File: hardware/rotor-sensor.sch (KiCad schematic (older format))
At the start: 47 parts, among them J1 Conn_01x03, J2 Conn_01x03, U1 EE-SX199, U2 MCP2021A-xxxxSN, U3 SM351LT, U4 ATtiny202-SS, U5 AP22804AW5

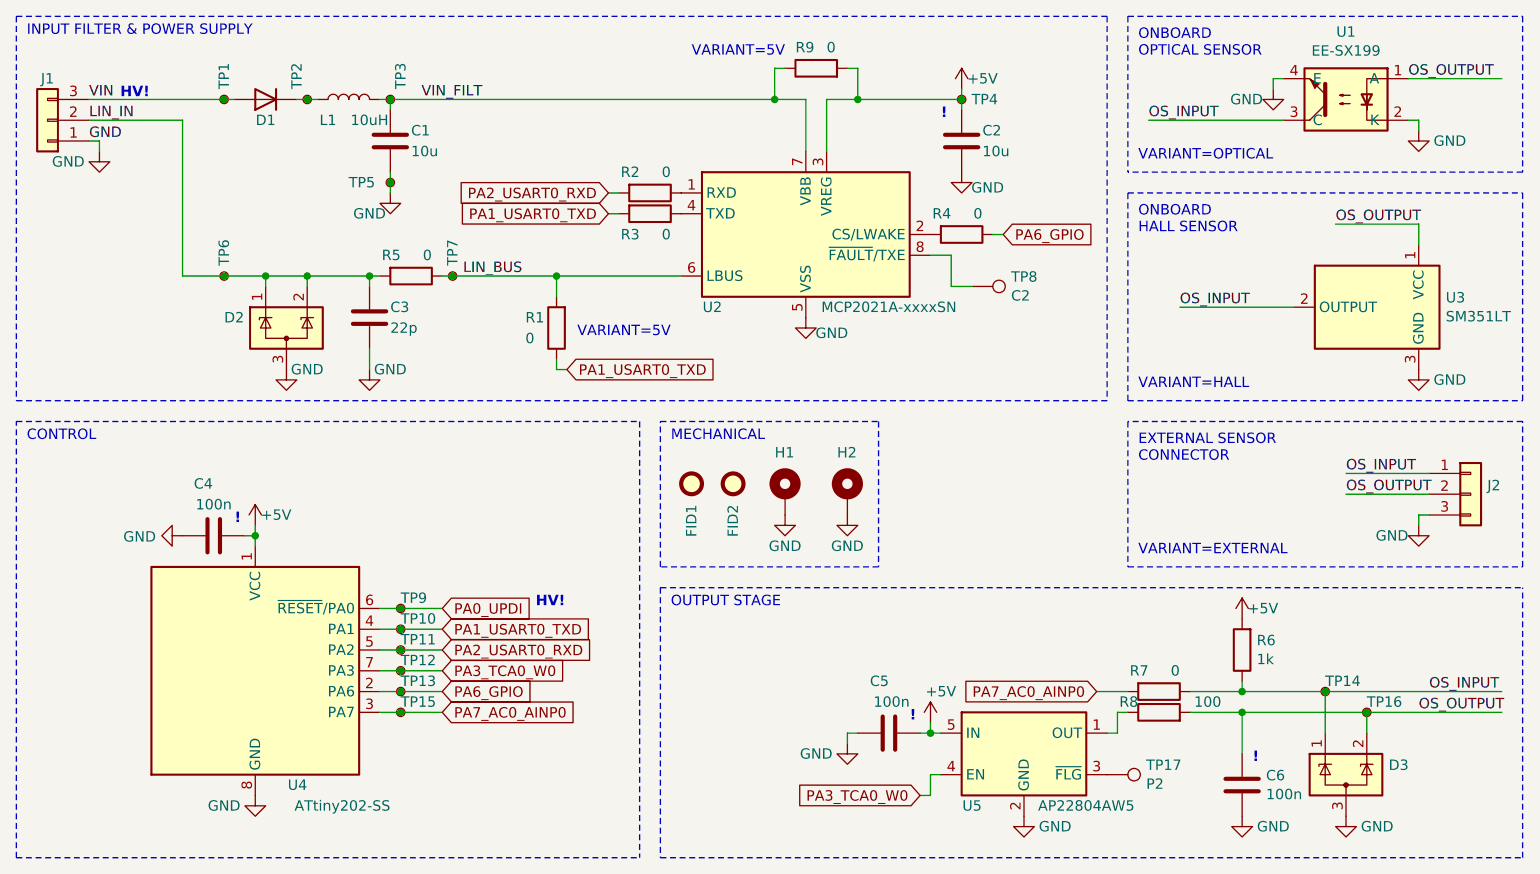
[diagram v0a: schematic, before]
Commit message: Panelize?
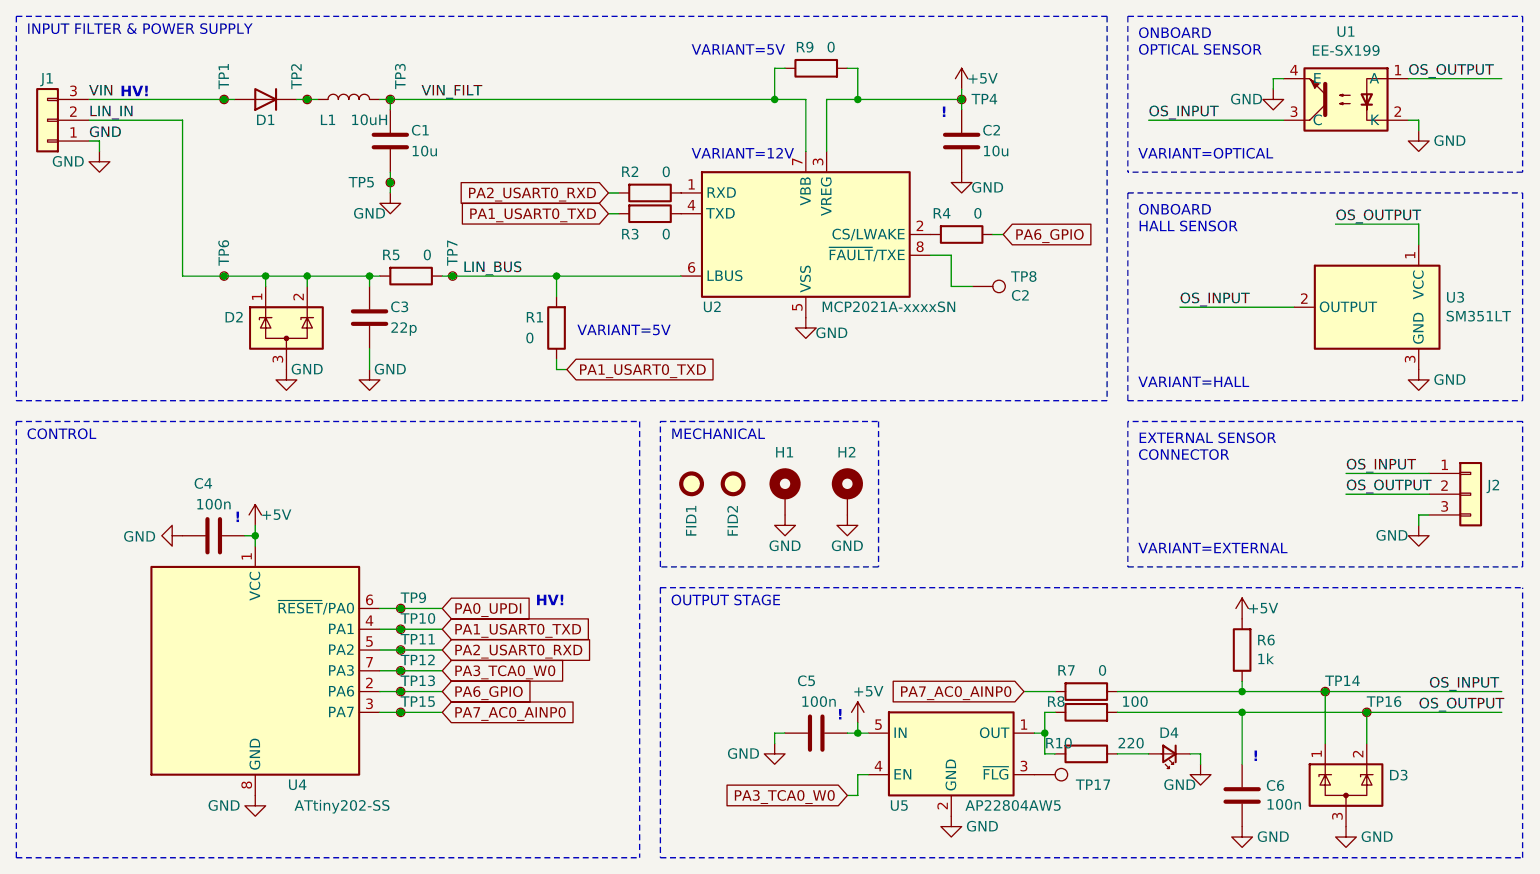
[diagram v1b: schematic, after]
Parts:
- added D4: LED_Small, LED_SMD:LED_0603_1608Metric, symbol Device:LED_Small
- added R10: 220, Resistor_SMD:R_0603_1608Metric, symbol Device:R
- R1, R9: Config (none) -> +5V
- U2: Config (none) -> -5V
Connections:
- wire segments 95 -> 100
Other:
- note added: "VARIANT=12V"
- moved on the sheet: C5, C6, D3, R7, R8, TP17, U5
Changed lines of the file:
@@
 L Device:R R8
 U 1 1 6122E61F
-P 7800 5100
-F 0 "R8" V 7850 5200 50  0000 L CNN
-F 1 "100" V 7850 4800 50  0000 L CNN
-F 2 "Resistor_SMD:R_0603_1608Metric" V 7730 5100 50  0001 C CNN
-F 3 "~" H 7800 5100 50  0001 C CNN
-	1    7800 5100
+P 7450 5100
+F 0 "R8" V 7500 5200 50  0000 L CNN
+F 1 "100" V 7500 4800 50  0000 L CNN
+F 2 "Resistor_SMD:R_0603_1608Metric" V 7380 5100 50  0001 C CNN
+F 3 "~" H 7450 5100 50  0001 C CNN
+	1    7450 5100
 	0    -1   -1   0
 $EndComp
@@
 	-1   0    0    1
 $EndComp
-Text GLabel 7500 5000 0    50   Input ~ 0
+Text GLabel 7150 5000 0    50   Input ~ 0
 PA7_AC0_AINP0
 Wire Wire Line
-	7600 5100 7650 5100
+	7250 5100 7300 5100
 Text GLabel 4350 4700 2    50   Input ~ 0
 PA1_USART0_TXD
@@
 L Power_Protection:SP0502BAHT D3
 U 1 1 613650DD
-P 8700 5400
-F 0 "D3" H 8905 5446 50  0000 L CNN
-F 1 "SP0502BAHT" H 8900 5350 50  0001 L CNN
-F 2 "Package_TO_SOT_SMD:SOT-23" H 8925 5350 50  0001 L CNN
-F 3 "http://www.littelfuse.com/~/media/files/littelfuse/technical%20resources/documents/data%20sheets/sp05xxba.pdf" H 8825 5525 50  0001 C CNN
-	1    8700 5400
+P 8700 5450
+F 0 "D3" H 8905 5496 50  0000 L CNN
+F 1 "SP0502BAHT" H 8900 5400 50  0001 L CNN
+F 2 "Package_TO_SOT_SMD:SOT-23" H 8925 5400 50  0001 L CNN
+F 3 "http://www.littelfuse.com/~/media/files/littelfuse/technical%20resources/documents/data%20sheets/sp05xxba.pdf" H 8825 5575 50  0001 C CNN
+	1    8700 5450
 	1    0    0    -1
 $EndComp
@@
 	8200 4950 8200 5000
 Wire Wire Line
-	8200 5300 8200 5100
+	8200 5350 8200 5100
 $Comp
 L power:GND #PWR024
 U 1 1 613B542D
-P 8700 5600
-F 0 "#PWR024" H 8700 5350 50  0001 C CNN
-F 1 "GND" H 8850 5550 50  0000 C CNN
-F 2 "" H 8700 5600 50  0001 C CNN
-F 3 "" H 8700 5600 50  0001 C CNN
-	1    8700 5600
+P 8700 5650
+F 0 "#PWR024" H 8700 5400 50  0001 C CNN
+F 1 "GND" H 8850 5600 50  0000 C CNN
+F 2 "" H 8700 5650 50  0001 C CNN
+F 3 "" H 8700 5650 50  0001 C CNN
+	1    8700 5650
 	1    0    0    -1
 $EndComp
@@
 L power:GND #PWR023
 U 1 1 6127F551
-P 8200 5600
-F 0 "#PWR023" H 8200 5350 50  0001 C CNN
-F 1 "GND" H 8350 5550 50  0000 C CNN
-F 2 "" H 8200 5600 50  0001 C CNN
-F 3 "" H 8200 5600 50  0001 C CNN
-	1    8200 5600
+P 8200 5650
+F 0 "#PWR023" H 8200 5400 50  0001 C CNN
+F 1 "GND" H 8350 5600 50  0000 C CNN
+F 2 "" H 8200 5650 50  0001 C CNN
+F 3 "" H 8200 5650 50  0001 C CNN
+	1    8200 5650
 	1    0    0    -1
 $EndComp
@@
 L Device:C C6
 U 1 1 61263E24
-P 8200 5450
-F 0 "C6" H 8315 5496 50  0000 L CNN
-F 1 "100n" H 8315 5405 50  0000 L CNN
-F 2 "Capacitor_SMD:C_0603_1608Metric" H 8238 5300 50  0001 C CNN
-F 3 "~" H 8200 5450 50  0001 C CNN
-	1    8200 5450
+P 8200 5500
+F 0 "C6" H 8315 5546 50  0000 L CNN
+F 1 "100n" H 8315 5455 50  0000 L CNN
+F 2 "Capacitor_SMD:C_0603_1608Metric" H 8238 5350 50  0001 C CNN
+F 3 "~" H 8200 5500 50  0001 C CNN
+	1    8200 5500
 	1    0    0    -1
 $EndComp
@@
 OUTPUT STAGE
 Wire Wire Line
-	8200 5000 7950 5000
-Wire Wire Line
-	7650 5000 7500 5000
+	8200 5000 7600 5000
+Wire Wire Line
+	7300 5000 7150 5000
 Text GLabel 4350 4600 2    50   Input ~ 0
 PA0_UPDI
@@
 	8350 2050 8400 2050
 Wire Wire Line
-	8800 5200 8800 5100
+	8800 5250 8800 5100
 Connection ~ 8800 5100
 Wire Wire Line
-	8600 5200 8600 5000
+	8600 5250 8600 5000
 Connection ~ 8600 5000
 Wire Wire Line
@@
 F 2 "Package_SO:SOIC-8_3.9x4.9mm_P1.27mm" H 6125 2875 50  0001 C CNN
 F 3 "http://ww1.microchip.com/downloads/en/DeviceDoc/20002298C.pdf" H 6125 2875 50  0001 C CNN
+F 4 "-5V" H 6100 2800 50  0001 C CNN "Config"
 	1    6100 2800
 	1    0    0    -1
@@
 Text GLabel 4350 4800 2    50   Input ~ 0
 PA2_USART0_RXD
-Wire Wire Line
-	7950 5100 8200 5100
 $Comp
 L Power_Management:AP22804AW5 U5
 U 1 1 623B800F
-P 7150 5300
-F 0 "U5" H 6900 5050 50  0000 C CNN
-F 1 "AP22804AW5" H 7450 5050 50  0000 C CNN
-F 2 "Package_TO_SOT_SMD:SOT-23-5" H 7150 4900 50  0001 C CNN
-F 3 "https://www.diodes.com/assets/Datasheets/AP22804_14.pdf" H 7150 5350 50  0001 C CNN
-	1    7150 5300
+P 6800 5300
+F 0 "U5" H 6550 5050 50  0000 C CNN
+F 1 "AP22804AW5" H 7100 5050 50  0000 C CNN
+F 2 "Package_TO_SOT_SMD:SOT-23-5" H 6800 4900 50  0001 C CNN
+F 3 "https://www.diodes.com/assets/Datasheets/AP22804_14.pdf" H 6800 5350 50  0001 C CNN
+	1    6800 5300
 	1    0    0    -1
 $EndComp
@@
 	5150 2700 5200 2700
 Wire Wire Line
-	7550 5200 7600 5200
-Wire Wire Line
-	7600 5200 7600 5100
+	7200 5200 7250 5200
+Wire Wire Line
+	7250 5200 7250 5100
 Text GLabel 4350 4900 2    50   Input ~ 0
 PA3_TCA0_W0
 Text GLabel 4350 5000 2    50   Input ~ 0
 PA6_GPIO
-Text GLabel 6650 5500 0    50   Input ~ 0
+Text GLabel 6300 5500 0    50   Input ~ 0
 PA3_TCA0_W0
 $Comp
 L power:+5V #PWR019
 U 1 1 623E7E3D
-P 6700 5150
-F 0 "#PWR019" H 6700 5000 50  0001 C CNN
-F 1 "+5V" H 6750 5300 50  0000 C CNN
-F 2 "" H 6700 5150 50  0001 C CNN
-F 3 "" H 6700 5150 50  0001 C CNN
-	1    6700 5150
-	1    0    0    -1
-$EndComp
-Wire Wire Line
-	6700 5400 6750 5400
-Wire Wire Line
-	6700 5150 6700 5200
-Wire Wire Line
-	6700 5200 6750 5200
+P 6350 5150
+F 0 "#PWR019" H 6350 5000 50  0001 C CNN
+F 1 "+5V" H 6400 5300 50  0000 C CNN
+F 2 "" H 6350 5150 50  0001 C CNN
+F 3 "" H 6350 5150 50  0001 C CNN
+	1    6350 5150
+	1    0    0    -1
+$EndComp
+Wire Wire Line
+	6350 5400 6400 5400
+Wire Wire Line
+	6350 5150 6350 5200
+Wire Wire Line
+	6350 5200 6400 5200
 $Comp
 L power:GND #PWR022
 U 1 1 623F4191
-P 7150 5600
-F 0 "#PWR022" H 7150 5350 50  0001 C CNN
-F 1 "GND" H 7300 5550 50  0000 C CNN
-F 2 "" H 7150 5600 50  0001 C CNN
-F 3 "" H 7150 5600 50  0001 C CNN
-	1    7150 5600
+P 6800 5600
+F 0 "#PWR022" H 6800 5350 50  0001 C CNN
+F 1 "GND" H 6950 5550 50  0000 C CNN
+F 2 "" H 6800 5600 50  0001 C CNN
+F 3 "" H 6800 5600 50  0001 C CNN
+	1    6800 5600
 	1    0    0    -1
 $EndComp
@@
 L Device:C C5
 U 1 1 623F6E9E
-P 6500 5200
-F 0 "C5" V 6750 5200 50  0000 L CNN
-F 1 "100n" V 6650 5100 50  0000 L CNN
-F 2 "Capacitor_SMD:C_0603_1608Metric" H 6538 5050 50  0001 C CNN
-F 3 "~" H 6500 5200 50  0001 C CNN
-	1    6500 5200
+P 6150 5200
+F 0 "C5" V 6400 5200 50  0000 L CNN
+F 1 "100n" V 6300 5100 50  0000 L CNN
+F 2 "Capacitor_SMD:C_0603_1608Metric" H 6188 5050 50  0001 C CNN
+F 3 "~" H 6150 5200 50  0001 C CNN
+	1    6150 5200
 	0    -1   -1   0
 $EndComp
@@
 L power:GND #PWR020
 U 1 1 6248AFD5
-P 6300 5250
-F 0 "#PWR020" H 6300 5000 50  0001 C CNN
-F 1 "GND" H 6150 5200 50  0000 C CNN
-F 2 "" H 6300 5250 50  0001 C CNN
-F 3 "" H 6300 5250 50  0001 C CNN
-	1    6300 5250
-	1    0    0    -1
-$EndComp
-Wire Wire Line
-	6650 5500 6700 5500
-Wire Wire Line
-	6700 5500 6700 5400
-Wire Wire Line
-	6300 5250 6300 5200
+P 5950 5250
+F 0 "#PWR020" H 5950 5000 50  0001 C CNN
+F 1 "GND" H 5800 5200 50  0000 C CNN
+F 2 "" H 5950 5250 50  0001 C CNN
+F 3 "" H 5950 5250 50  0001 C CNN
+	1    5950 5250
+	1    0    0    -1
+$EndComp
+Wire Wire Line
+	6300 5500 6350 5500
+Wire Wire Line
+	6350 5500 6350 5400
+Wire Wire Line
+	5950 5250 5950 5200
+Wire Wire Line
+	5950 5200 6000 5200
 Wire Wire Line
 	6300 5200 6350 5200
-Wire Wire Line
-	6650 5200 6700 5200
-Connection ~ 6700 5200
+Connection ~ 6350 5200
 Wire Notes Line
 	5400 4500 9550 4500
@@
 L Device:R R7
 U 1 1 6258FF8B
-P 7800 5000
-F 0 "R7" V 7700 4950 50  0000 R CNN
-F 1 "0" V 7700 5100 50  0000 R CNN
-F 2 "Resistor_SMD:R_0402_1005Metric" V 7730 5000 50  0001 C CNN
-F 3 "~" H 7800 5000 50  0001 C CNN
-	1    7800 5000
+P 7450 5000
+F 0 "R7" V 7350 4950 50  0000 R CNN
+F 1 "0" V 7350 5100 50  0000 R CNN
+F 2 "Resistor_SMD:R_0402_1005Metric" V 7380 5000 50  0001 C CNN
+F 3 "~" H 7450 5000 50  0001 C CNN
+	1    7450 5000
 	0    1    1    0
 $EndComp
@@
 L Connector:TestPoint TP17
 U 1 1 626156D9
-P 7550 5400
-F 0 "TP17" V 7504 5588 50  0000 L CNN
-F 1 "P2" V 7595 5588 50  0000 L CNN
-F 2 "TestPoint:TestPoint_Pad_D1.0mm" H 7750 5400 50  0001 C CNN
-F 3 "~" H 7750 5400 50  0001 C CNN
-	1    7550 5400
+P 7200 5400
+F 0 "TP17" V 7250 5600 50  0000 L CNN
+F 1 "P2" V 7300 5600 50  0001 L CNN
+F 2 "TestPoint:TestPoint_Pad_D1.0mm" H 7400 5400 50  0001 C CNN
+F 3 "~" H 7400 5400 50  0001 C CNN
+	1    7200 5400
 	0    1    1    0
 $EndComp
@@
 Text Label 8650 2750 0    50   ~ 0
 OS_OUTPUT
-Text Notes 6600 5150 0    50   ~ 10
+Text Notes 6250 5150 0    50   ~ 10
 !
 Text Notes 6750 2250 0    50   ~ 10
@@
 F 2 "Resistor_SMD:R_0402_1005Metric" V 4830 3250 50  0001 C CNN
 F 3 "~" H 4900 3250 50  0001 C CNN
+F 4 "+5V" H 4900 3250 50  0001 C CNN "Config"
 	1    4900 3250
 	-1   0    0    1
@@
 F 2 "Resistor_SMD:R_0603_1608Metric" V 6080 2000 50  0001 C CNN
 F 3 "~" H 6150 2000 50  0001 C CNN
+F 4 "+5V" V 6150 2000 50  0001 C CNN "Config"
 	1    6150 2000
 	0    -1   -1   0
@@
 Text Notes 5000 3300 0    50   ~ 0
 VARIANT=5V
+$Comp
+L Device:R R10
+U 1 1 6253E802
+P 7450 5300
+F 0 "R10" V 7400 5100 50  0000 L CNN
+F 1 "220" V 7400 5450 50  0000 L CNN
+F 2 "Resistor_SMD:R_0603_1608Metric" V 7380 5300 50  0001 C CNN
+F 3 "~" H 7450 5300 50  0001 C CNN
+	1    7450 5300
+	0    1    1    0
+$EndComp
+$Comp
+L Device:LED_Small D4
+U 1 1 6253FA73
+P 7850 5300
+F 0 "D4" H 7900 5200 50  0000 R CNN
+F 1 "LED_Small" V 7800 5500 50  0001 R CNN
+F 2 "LED_SMD:LED_0603_1608Metric" V 7850 5300 50  0001 C CNN
+F 3 "~" V 7850 5300 50  0001 C CNN
+	1    7850 5300
+	-1   0    0    1
+$EndComp
+$Comp
+L power:GND #PWR0101
+U 1 1 625403F5
+P 8000 5350
+F 0 "#PWR0101" H 8000 5100 50  0001 C CNN
+F 1 "GND" H 7900 5250 50  0000 C CNN
+F 2 "" H 8000 5350 50  0001 C CNN
+F 3 "" H 8000 5350 50  0001 C CNN
+	1    8000 5350
+	1    0    0    -1
+$EndComp
+Wire Wire Line
+	7600 5100 8200 5100
+Wire Wire Line
+	7250 5200 7250 5300
+Wire Wire Line
+	7250 5300 7300 5300
+Connection ~ 7250 5200
+Wire Wire Line
+	7950 5300 8000 5300
+Wire Wire Line
+	8000 5300 8000 5350
+Wire Wire Line
+	7600 5300 7750 5300
+Text Notes 5550 2450 0    50   ~ 0
+VARIANT=12V
 $EndSCHEMATC
